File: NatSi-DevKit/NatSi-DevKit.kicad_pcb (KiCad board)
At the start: 4 copper layers, 25.4 x 62.5 mm, 47 parts, among them J1 USB_TypeC, J2 Conn_01x22_Pin, J3 Conn_01x22_Pin, J4 MEM2067-02-180-00-A_REVB, SW1 SW_Push, SW2 SW_Push, SW3 SW_Push, U1 USBLC6-2SC6, U2 ESP32-S3-WROOM-1, U3 NCP1117-3.3_SOT223

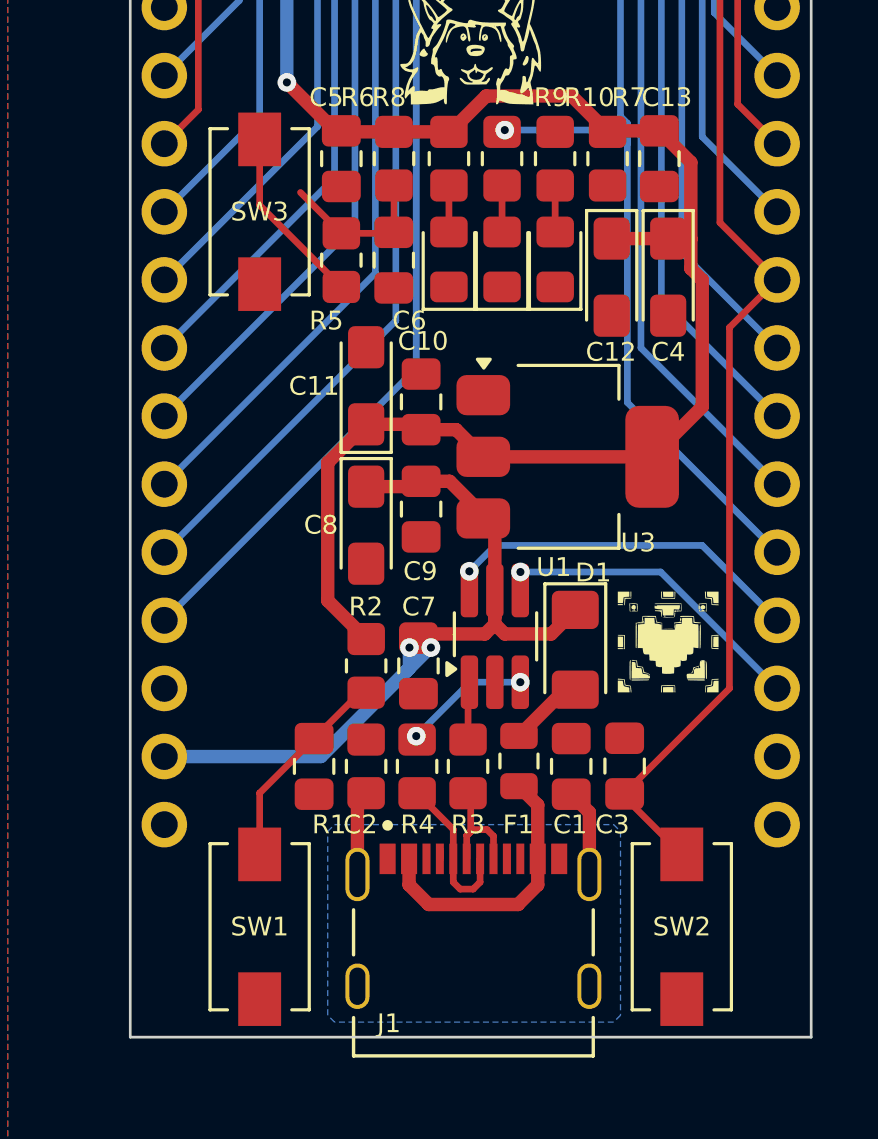
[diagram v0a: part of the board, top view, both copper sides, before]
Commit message: some 3d updates
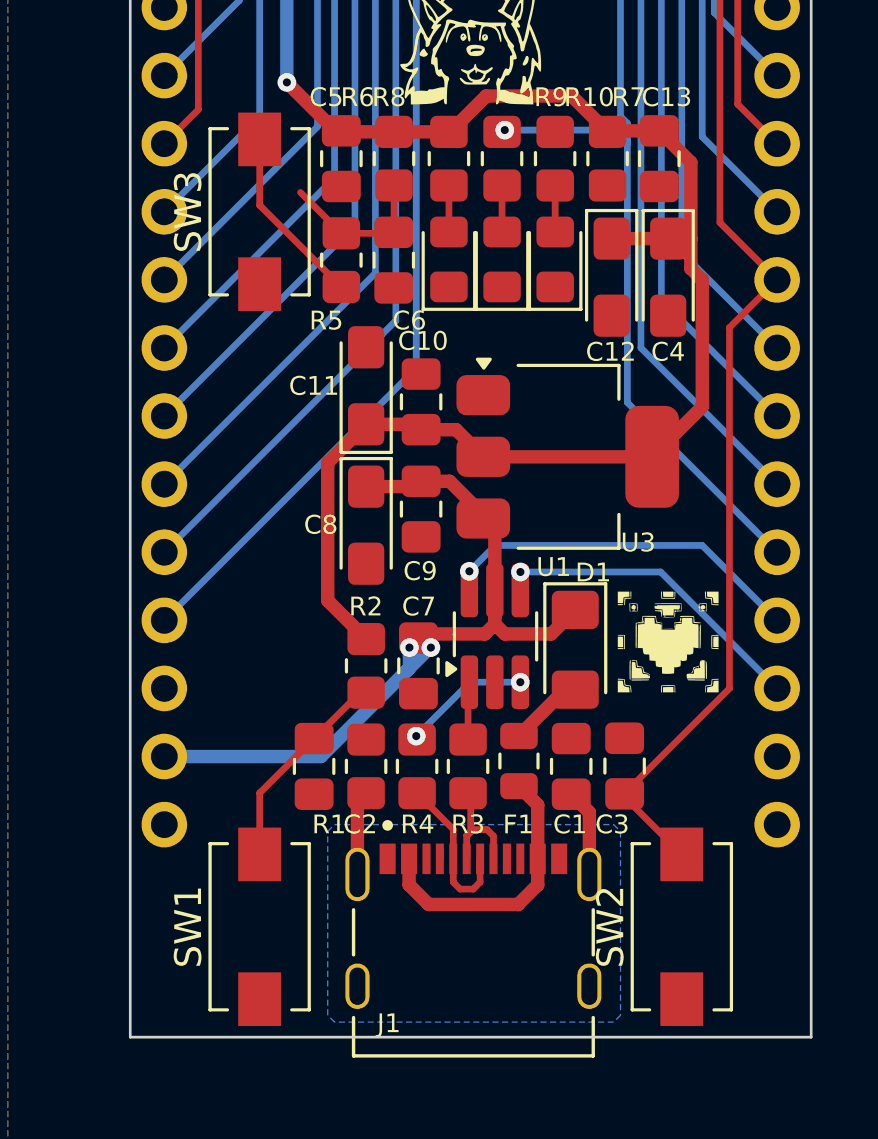
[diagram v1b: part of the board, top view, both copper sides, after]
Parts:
- SW1, SW2, SW3: footprint Button_Switch_SMD:SW_SPST_EVQPE1 -> sumec_brd:SW_SPST_EVQPE1
